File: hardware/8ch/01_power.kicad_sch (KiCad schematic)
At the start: 0 parts

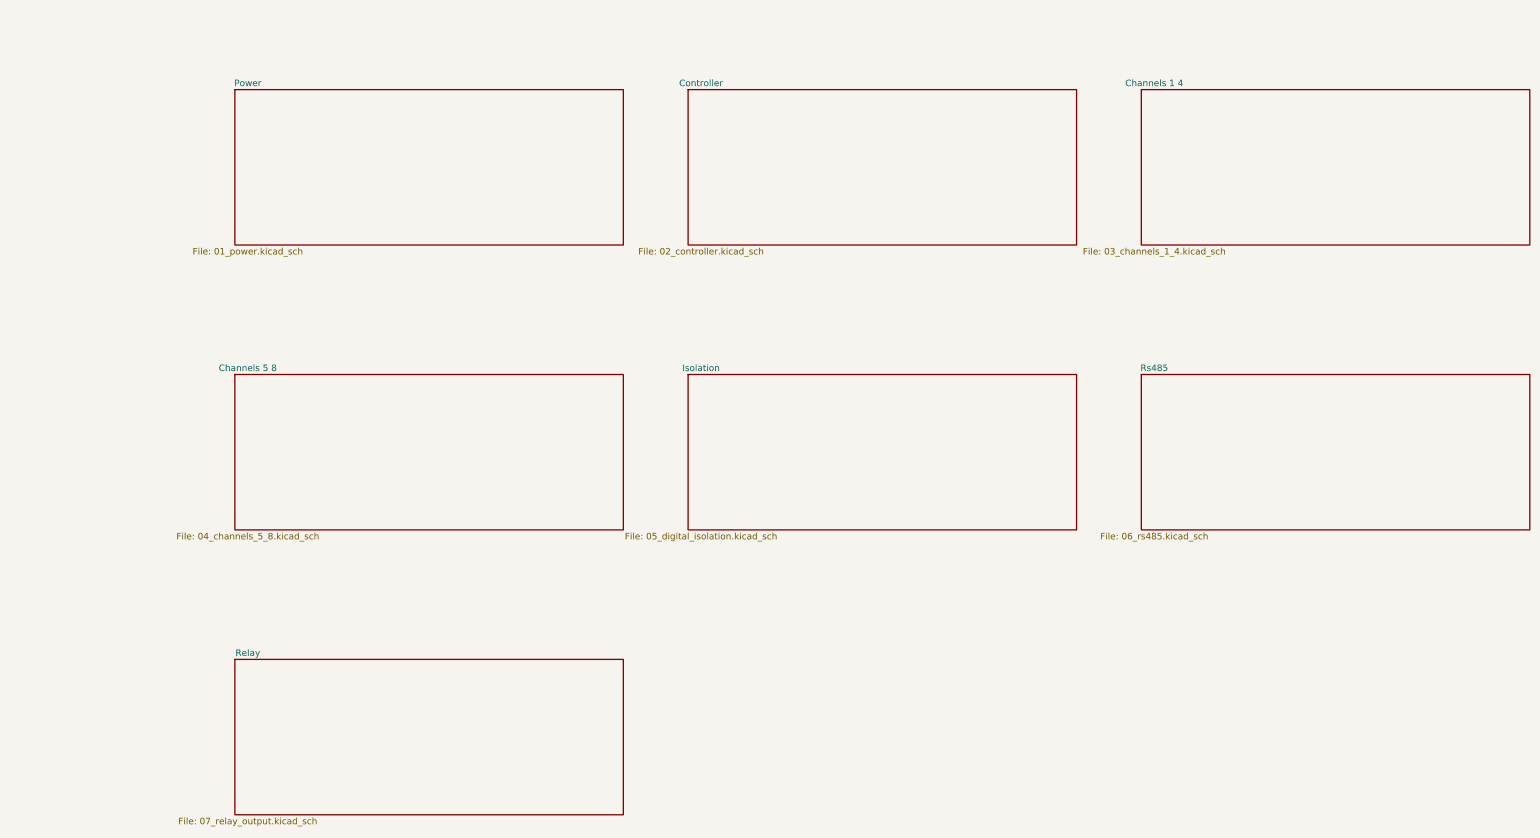
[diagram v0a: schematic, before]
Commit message: fix bugs
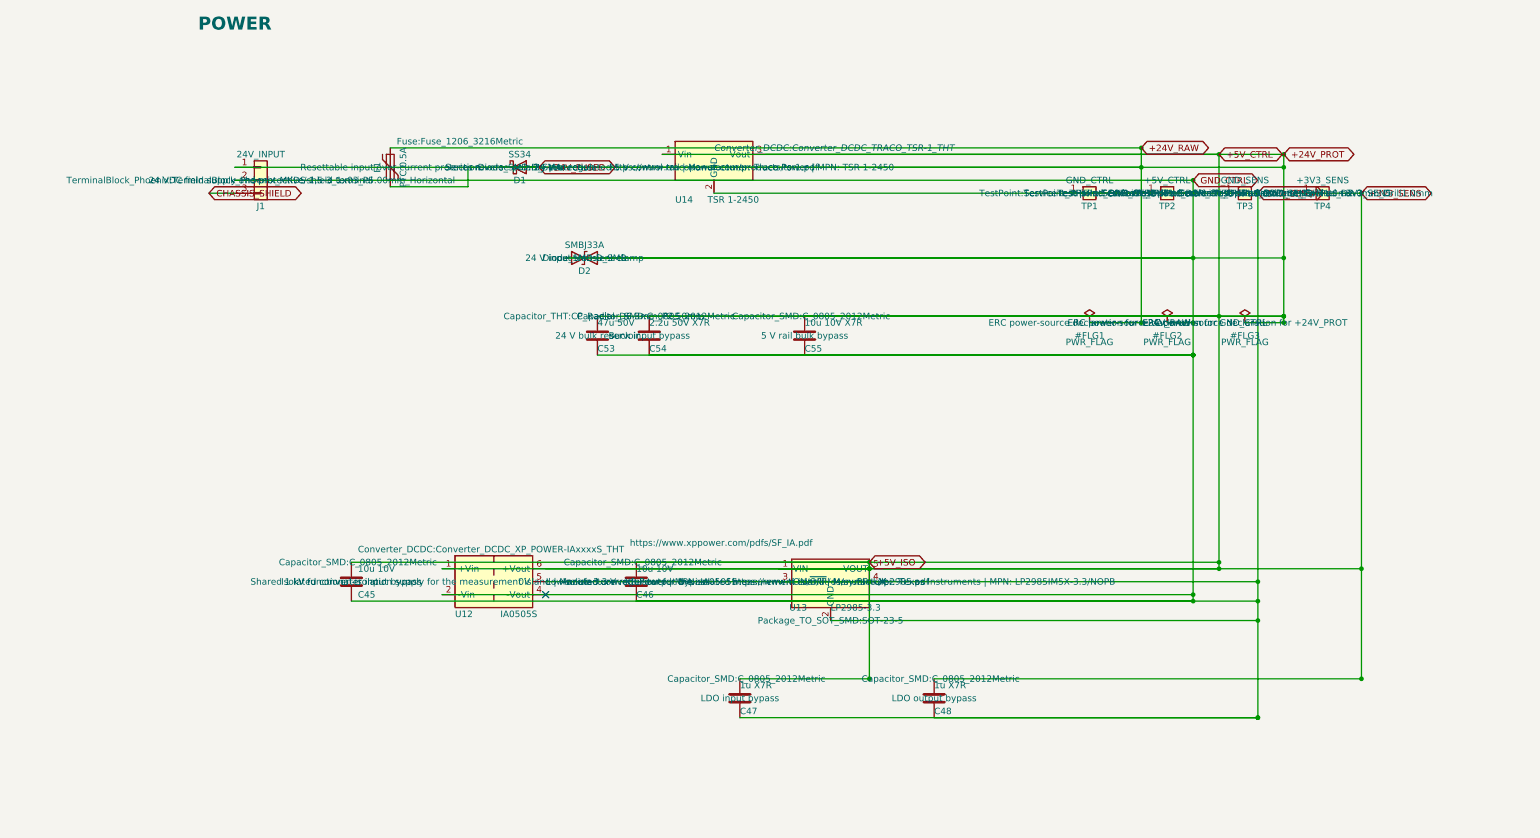
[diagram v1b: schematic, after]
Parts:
- added C45, C46: 10u 10V, Capacitor_SMD:C_0805_2012Metric, symbol Device:C
- added C47, C48: 1u X7R, Capacitor_SMD:C_0805_2012Metric, symbol Device:C
- added C53: 47u 50V, Capacitor_THT:CP_Radial_D6.3mm_P2.50mm, symbol Device:C
- added C54: 2.2u 50V X7R, Capacitor_SMD:C_0805_2012Metric, symbol Device:C
- added C55: 10u 10V X7R, Capacitor_SMD:C_0805_2012Metric, symbol Device:C
- added D1: SS34, Diode_SMD:D_SMA, symbol Device:D_Schottky
- added D2: SMBJ33A, Diode_SMD:D_SMB, symbol Device:D_TVS
- added F1: PTC 0.5A, Fuse:Fuse_1206_3216Metric, symbol Device:Polyfuse
- added J1: 24V_INPUT, TerminalBlock_Phoenix:TerminalBlock_Phoenix_MKDS-1,5-3_1x03_P5.00mm_Horizontal, symbol Connector_Generic:Conn_01x03
- added TP1: GND_CTRL, TestPoint:TestPoint_THTPad_D2.0mm_Drill1.0mm, symbol Connector_Generic:Conn_01x01
- added TP2: +5V_CTRL, TestPoint:TestPoint_THTPad_D2.0mm_Drill1.0mm, symbol Connector_Generic:Conn_01x01
- added TP3: GND_SENS, TestPoint:TestPoint_THTPad_D2.0mm_Drill1.0mm, symbol Connector_Generic:Conn_01x01
- added TP4: +3V3_SENS, TestPoint:TestPoint_THTPad_D2.0mm_Drill1.0mm, symbol Connector_Generic:Conn_01x01
- added U12: IA0505S, Converter_DCDC:Converter_DCDC_XP_POWER-IAxxxxS_THT, symbol Converter_DCDC:IA0305S
- added U13: LP2985-3.3, Package_TO_SOT_SMD:SOT-23-5, symbol Regulator_Linear:LP2985-1.8
- added U14: TSR 1-2450, Converter_DCDC:Converter_DCDC_TRACO_TSR-1_THT, symbol Converter_DCDC:TSR_1-2450
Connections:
- new net +24V_FUSED: C45.1, C45.2, C46.1, C46.2, C47.1, C47.2, C48.1, C48.2, C53.1, C53.2, C54.1, C54.2, C55.1, C55.2, D1.1 (K), D1.2 (A), D2.1 (A1), D2.2 (A2), F1.1, F1.2, J1.1 (Pin_1), J1.2 (Pin_2), TP1.1 (Pin_1), TP2.1 (Pin_1), TP3.1 (Pin_1), TP4.1 (Pin_1), U12.1 (+Vin), U12.2 (-Vin), U12.5 (0V), U12.6 (+Vout), U13.1 (VIN), U13.2 (GND), U13.3 (ON/~{OFF}), U13.5 (VOUT), U14.1 (Vin), U14.2 (GND), U14.3 (Vout)
- new net CHASSIS_SHIELD: J1.3 (Pin_3)
- no-connect marks 0 -> 2
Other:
- removed sheet Channels 1 4
- removed sheet Channels 5 8
- removed sheet Controller
- removed sheet Isolation
- removed sheet Power
- removed sheet Relay
- removed sheet Rs485
- note added: "POWER"
